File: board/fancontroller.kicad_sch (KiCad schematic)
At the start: 6 parts, among them J1 Thermo

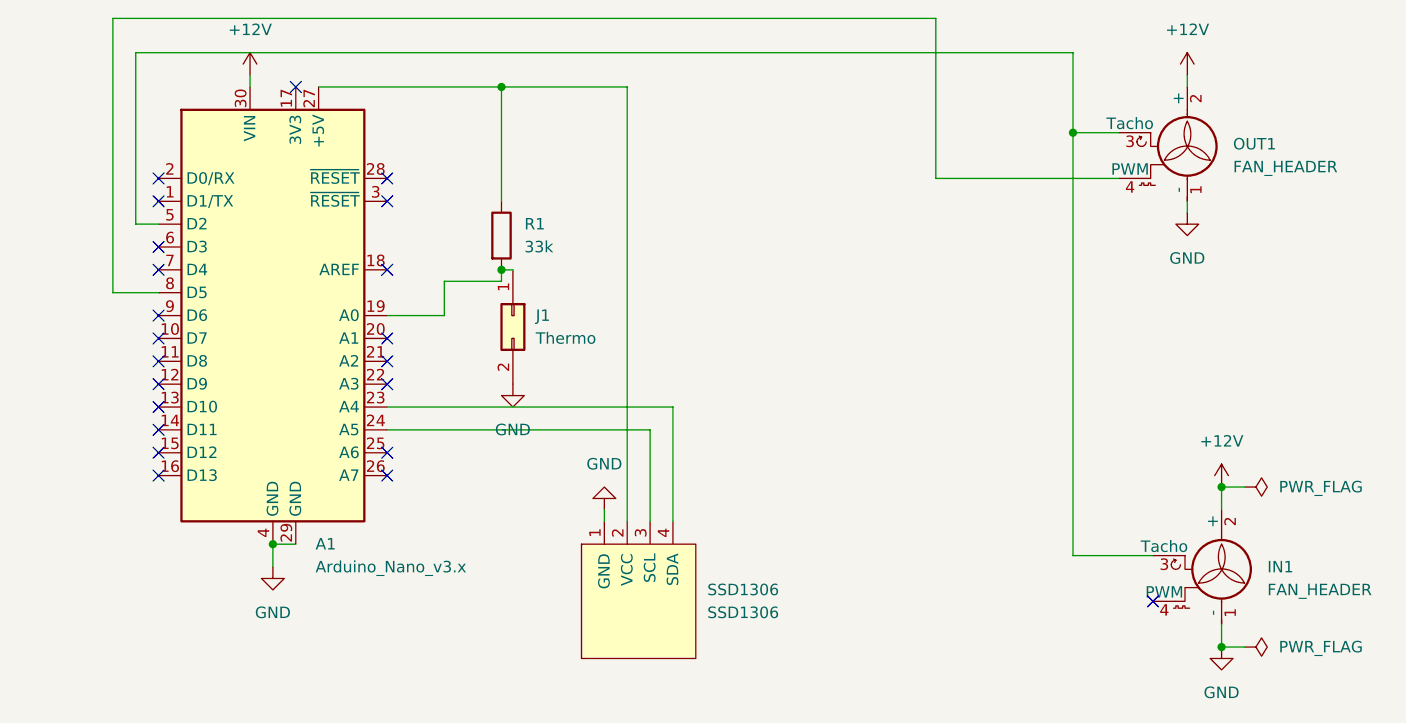
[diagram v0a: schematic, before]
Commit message: wip
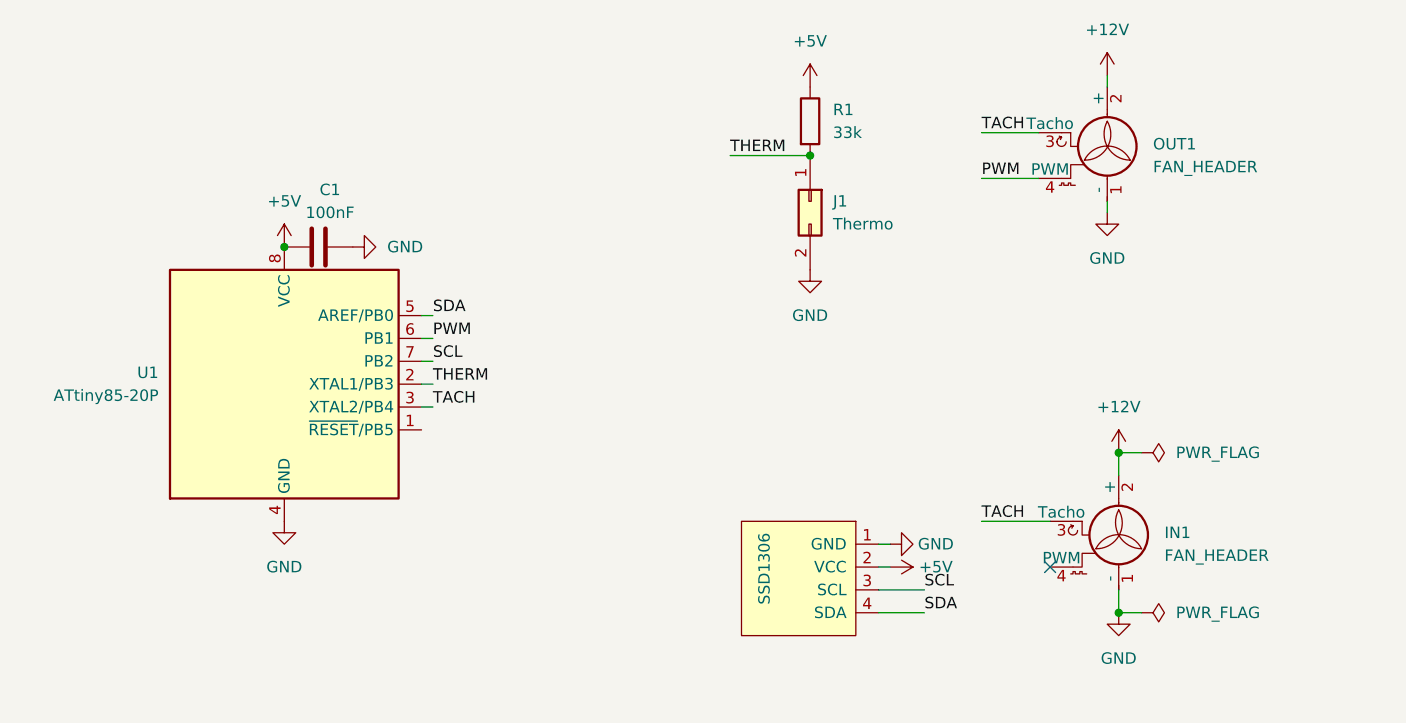
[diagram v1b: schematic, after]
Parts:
- removed A1: Arduino_Nano_v3.x, Module:Arduino_Nano, symbol MCU_Module:Arduino_Nano_v3.x
- added C1: 100nF, Capacitor_THT:C_Disc_D3.0mm_W1.6mm_P2.50mm, symbol Device:C
- added U1: ATtiny85-20P, Package_DIP:DIP-8_W7.62mm, symbol MCU_Microchip_ATtiny:ATtiny85-20P
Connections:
- net GND: now also C1.2, U1.4 (GND)
- net THERM: now reaches J1.1 (Pin_1), R1.2
- net THERM: now also U1.2 (XTAL1/PB3)
- net SDA: now reaches SSD1306.4 (SDA)
- net SDA: now also U1.5 (AREF/PB0)
- net SCL: now reaches SSD1306.3 (SCL)
- net SCL: now also U1.7 (PB2)
- net +5V: now reaches R1.1, SSD1306.2 (VCC)
- net +5V: now also C1.1, U1.8 (VCC)
- net TACH: now reaches IN1.3 (Tacho), OUT1.3 (Tacho)
- net TACH: now also U1.3 (XTAL2/PB4)
- net PWM: now reaches OUT1.4 (PWM)
- net PWM: now also U1.6 (PB1)
- no-connect marks 22 -> 1
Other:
- moved on the sheet: IN1, J1, OUT1, R1, SSD1306
